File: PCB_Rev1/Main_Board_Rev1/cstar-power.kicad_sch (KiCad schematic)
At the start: 49 parts, among them IC1 LT8648SEV#PBF, J4 Conn_01x02_Pin, J5 XT60PW-M, J6 Conn_01x02_Pin, J7 Conn_01x02_Pin, J8 Conn_01x02_Pin, U1 AZ1117IH-3.3TRG1

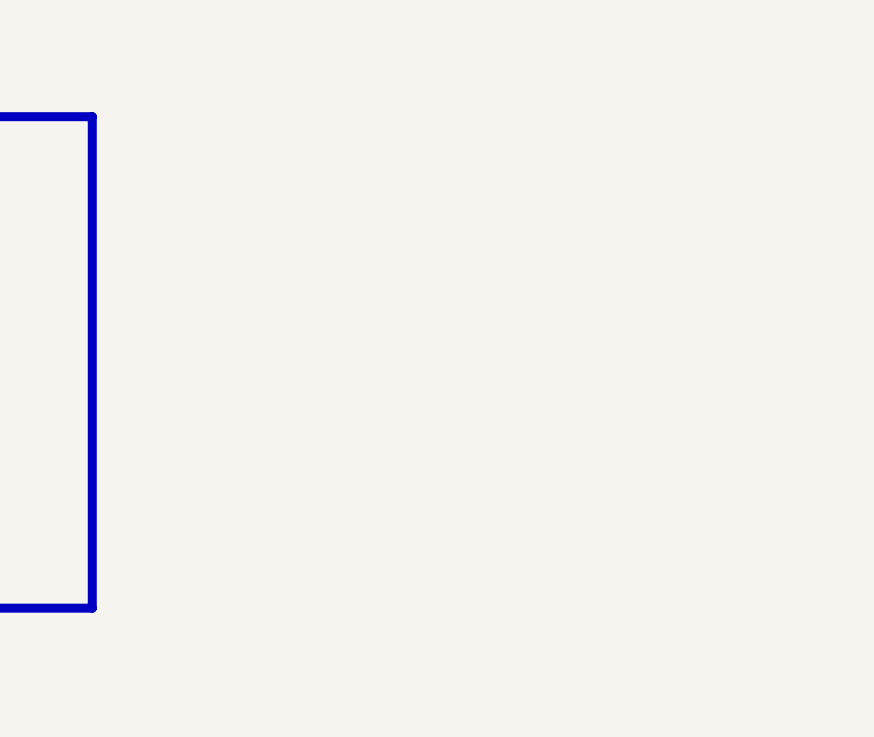
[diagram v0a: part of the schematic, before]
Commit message: deruioiygfhjik
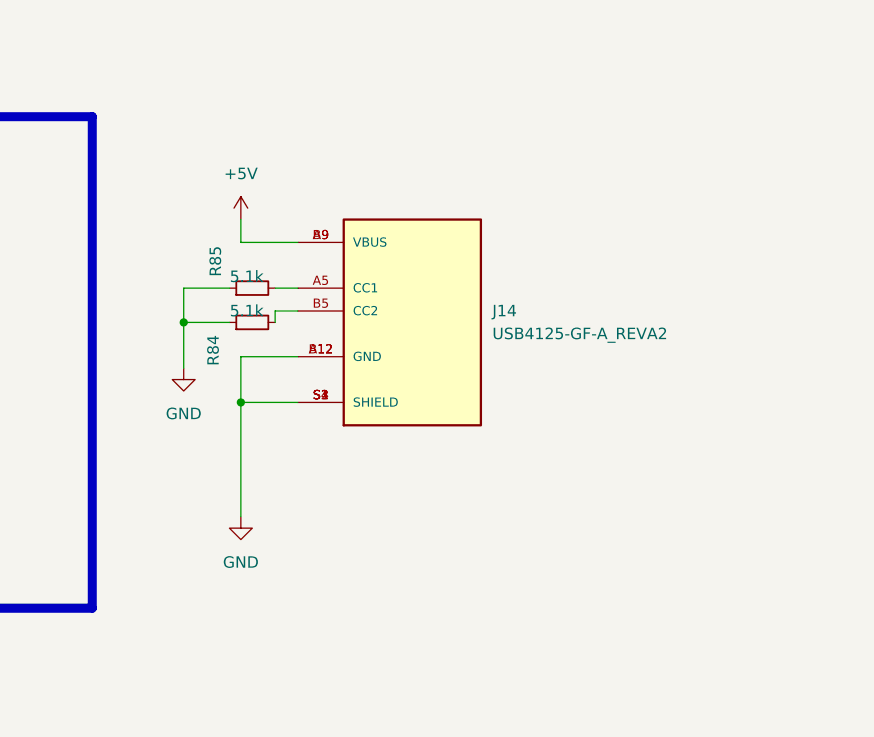
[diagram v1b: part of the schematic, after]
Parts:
- added J14: USB4125-GF-A_REVA2, Footprints:GCT_USB4125-GF-A_REVA2, symbol USB:USB4125-GF-A_REVA2
- added R84, R85: 5.1k, Resistor_SMD:R_0805_2012Metric, symbol Device:R_Small
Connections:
- net +5V: now also J14.A9 (VBUS), J14.B9 (VBUS)
- net GND: now also J14.A12 (GND), J14.B12 (GND), J14.S1 (SHIELD), J14.S2 (SHIELD), J14.S3 (SHIELD), J14.S4 (SHIELD), R84.1, R85.1
- new net: J14.A5 (CC1), R85.2
- new net: J14.B5 (CC2), R84.2
